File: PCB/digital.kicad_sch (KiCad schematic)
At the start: 29 parts, among them J14 FINAL_CARRERA_UP, J15 FINAL_CARRERA_DOWN, J3 ICSP, J4 CAN, J6 USART, J7 SPI, J8 RFID_COAX, U2 PIC32MK0256MCJ048-I/Y8X, U3 TCAN334D, Y1 ASZKDV-32.768KHZ-L-T3, Y2 ECS-3225SMV-080-GP-TR

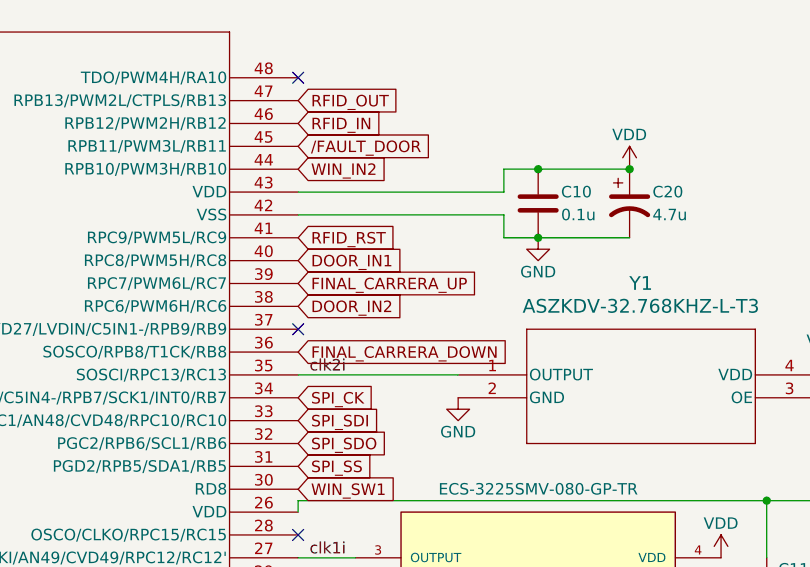
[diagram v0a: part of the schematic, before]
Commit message: canvis i arreglos
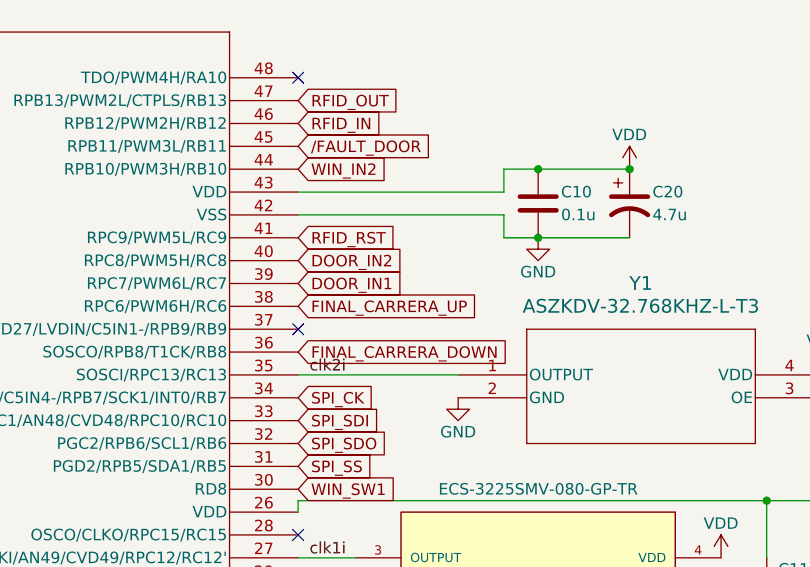
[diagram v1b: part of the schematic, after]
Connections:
- net DOOR_IN1: now also U2.39 (RPC7/PWM6L/RC7); no longer U2.40 (RPC8/PWM5H/RC8)
- net DOOR_IN2: now also U2.40 (RPC8/PWM5H/RC8); no longer U2.38 (RPC6/PWM6H/RC6)
- net FINAL_CARRERA_UP: now also U2.38 (RPC6/PWM6H/RC6); no longer U2.39 (RPC7/PWM6L/RC7)
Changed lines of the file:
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@@
+    )
+  )
+  (global_label "FINAL_CARRERA_UP" (shape input) (at 217.17 60.96 0) (fields_autoplaced)
+    (effects (font (size 1.27 1.27)) (justify left))
+    (property "Intersheetrefs" "${INTERSHEET_REFS}" (at 238.2377 60.96 0)
+      (effects (font (size 1.27 1.27)) (justify left) hide)
     )
   )
@@
     )
   )
-  (global_label "DOOR_IN2" (shape input) (at 217.17 60.96 0) (fields_autoplaced)
+  (global_label "{slash}MCLR" (shape input) (at 78.74 27.94 90) (fields_autoplaced)
     (effects (font (size 1.27 1.27)) (justify left))
-    (property "Intersheetrefs" "${INTERSHEET_REFS}" (at 229.3892 60.96 0)
+    (property "Intersheetrefs" "${INTERSHEET_REFS}" (at 78.74 18.6048 90)
       (effects (font (size 1.27 1.27)) (justify left) hide)
     )
   )
-  (global_label "{slash}MCLR" (shape input) (at 78.74 27.94 90) (fields_autoplaced)
+  (global_label "DOOR_IN2" (shape input) (at 217.17 55.88 0) (fields_autoplaced)
     (effects (font (size 1.27 1.27)) (justify left))
-    (property "Intersheetrefs" "${INTERSHEET_REFS}" (at 78.74 18.6048 90)
+    (property "Intersheetrefs" "${INTERSHEET_REFS}" (at 229.3892 55.88 0)
       (effects (font (size 1.27 1.27)) (justify left) hide)
     )
@@
     )
   )
+  (global_label "DOOR_IN1" (shape input) (at 217.17 58.42 0) (fields_autoplaced)
+    (effects (font (size 1.27 1.27)) (justify left))
+    (property "Intersheetrefs" "${INTERSHEET_REFS}" (at 229.3892 58.42 0)
+      (effects (font (size 1.27 1.27)) (justify left) hide)
+    )
+  )
   (global_label "CAN_RX" (shape input) (at 85.09 60.96 180) (fields_autoplaced)
     (effects (font (size 1.27 1.27)) (justify right))
@@
     (property "Intersheetrefs" "${INTERSHEET_REFS}" (at 304.5967 97.79 0)
       (effects (font (size 1.27 1.27)) (justify right) hide)
-    )
-  )
-  (global_label "FINAL_CARRERA_UP" (shape input) (at 217.17 58.42 0) (fields_autoplaced)
-    (effects (font (size 1.27 1.27)) (justify left))
-    (property "Intersheetrefs" "${INTERSHEET_REFS}" (at 238.2377 58.42 0)
-      (effects (font (size 1.27 1.27)) (justify left) hide)
     )
   )
@@
     )
   )
-  (global_label "DOOR_IN1" (shape input) (at 217.17 55.88 0) (fields_autoplaced)
-    (effects (font (size 1.27 1.27)) (justify left))
-    (property "Intersheetrefs" "${INTERSHEET_REFS}" (at 229.3892 55.88 0)
-      (effects (font (size 1.27 1.27)) (justify left) hide)
-    )
-  )
